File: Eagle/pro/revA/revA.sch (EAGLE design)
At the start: 57 parts, among them Q1 20MHz, U1 MCP42XXX

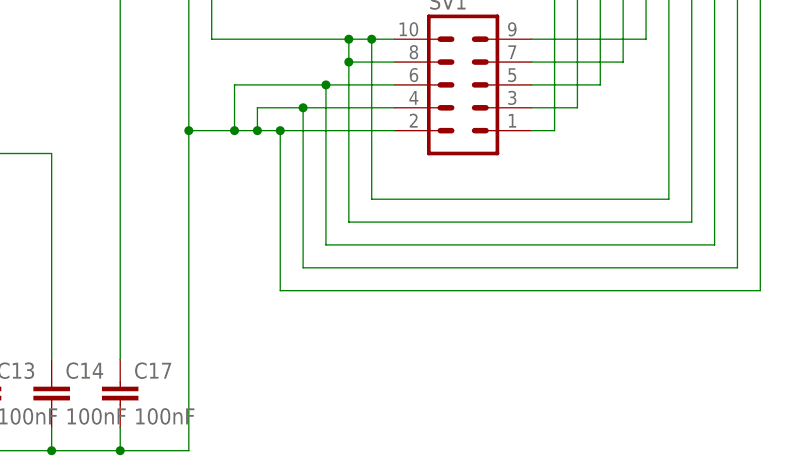
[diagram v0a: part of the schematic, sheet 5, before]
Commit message: silkscreen
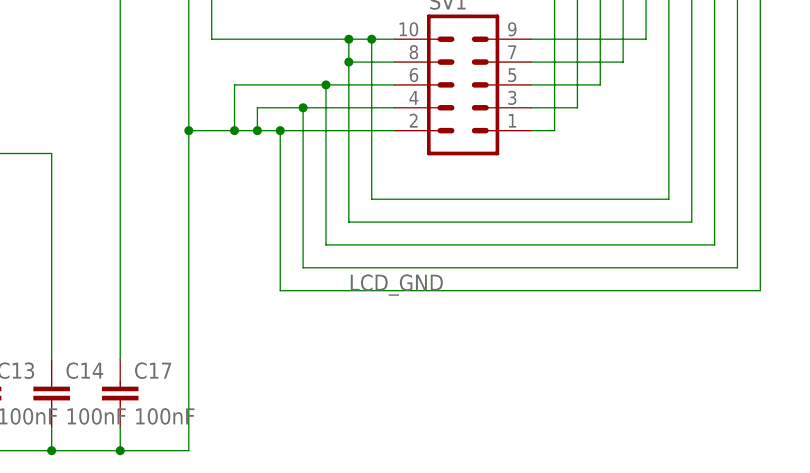
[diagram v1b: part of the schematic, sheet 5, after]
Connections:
- net N$22 renamed LCD_GND
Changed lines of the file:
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@@
 </segment>
 </net>
-<net name="N$22" class="0">
+<net name="LCD_GND" class="0">
 <segment>
 <pinref part="SV1" gate="G$1" pin="6"/>
@@
 <wire x1="76.2" y1="104.14" x2="76.2" y2="76.2" width="0.1524" layer="91"/>
 <junction x="76.2" y="76.2"/>
+<label x="93.98" y="58.42" size="1.778" layer="95"/>
 </segment>
 </net>
